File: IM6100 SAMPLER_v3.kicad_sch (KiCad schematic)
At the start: 0 parts

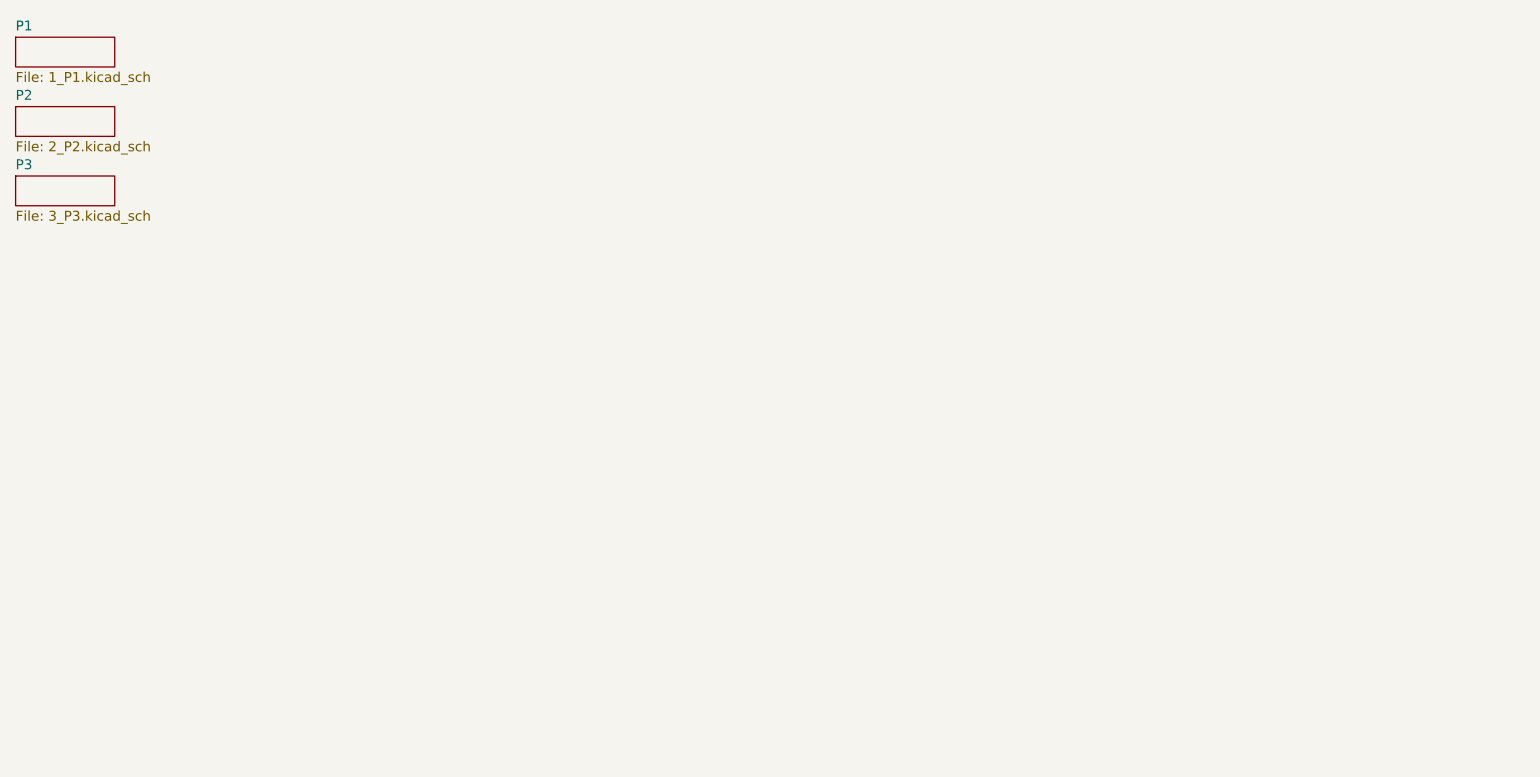
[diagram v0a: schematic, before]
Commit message: HID board finalizing
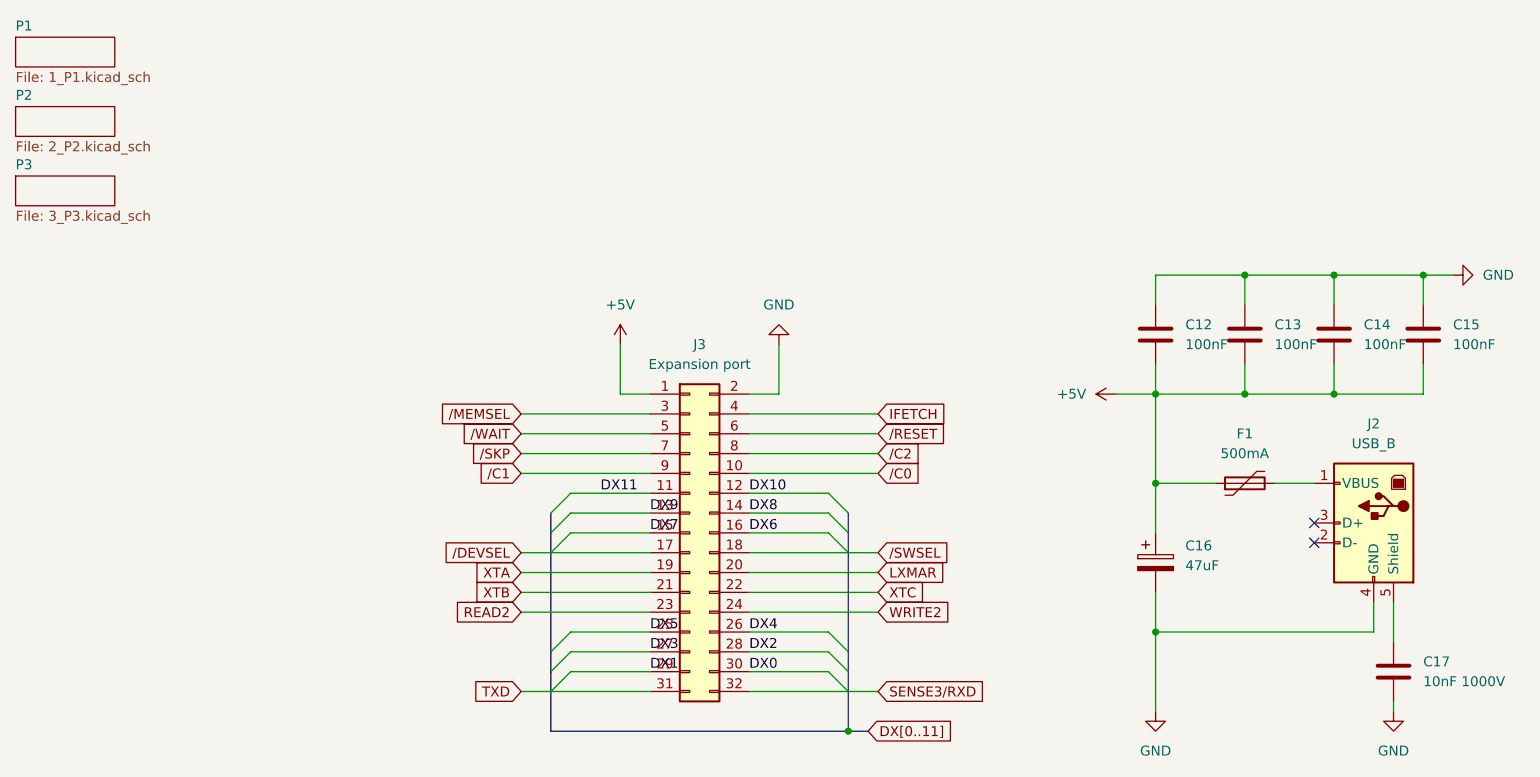
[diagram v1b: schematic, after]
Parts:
- added C12, C13, C14, C15: 100nF, Capacitor_THT:C_Disc_D5.0mm_W2.5mm_P2.50mm, symbol Device:C
- added C16: 47uF, Capacitor_THT:CP_Radial_D6.3mm_P2.50mm, symbol Device:C_Polarized
- added C17: 10nF 1000V, Capacitor_THT:C_Disc_D5.0mm_W2.5mm_P2.50mm, symbol Device:C
- added F1: 500mA, Capacitor_THT:C_Disc_D6.0mm_W2.5mm_P5.00mm, symbol Device:Polyfuse
- added J2: USB_B, Connector_USB:USB_B_Lumberg_2411_02_Horizontal, symbol Connector:USB_B
- added J3: Expansion port, Connector_PinHeader_2.54mm:PinHeader_2x16_P2.54mm_Vertical, symbol Connector_Generic:Conn_02x16_Odd_Even
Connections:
- new net: F1.2, J2.1 (VBUS)
- new net: C17.1, J2.5 (Shield)
- new net +5V: C12.2, C13.2, C14.2, C15.2, C16.1, F1.1, J3.1 (Pin_1)
- new net /C0: J3.10 (Pin_10)
- new net /C1: J3.9 (Pin_9)
- new net /C2: J3.8 (Pin_8)
- new net /DEVSEL: J3.17 (Pin_17)
- new net /MEMSEL: J3.3 (Pin_3)
- new net /SKP: J3.7 (Pin_7)
- new net /SWSEL: J3.18 (Pin_18)
- new net DX0: J3.30 (Pin_30)
- new net DX1: J3.29 (Pin_29)
- new net DX10: J3.12 (Pin_12)
- new net DX11: J3.11 (Pin_11)
- new net DX2: J3.28 (Pin_28)
- new net DX3: J3.27 (Pin_27)
- new net DX4: J3.26 (Pin_26)
- new net DX5: J3.25 (Pin_25)
- new net DX6: J3.16 (Pin_16)
- new net DX7: J3.15 (Pin_15)
- new net DX8: J3.14 (Pin_14)
- new net DX9: J3.13 (Pin_13)
- new net GND: C12.1, C13.1, C14.1, C15.1, C16.2, C17.2, J2.4 (GND), J3.2 (Pin_2)
- new net IFETCH: J3.4 (Pin_4)
- new net LXMAR: J3.20 (Pin_20)
- new net READ2: J3.23 (Pin_23)
- new net SENSE3/RXD: J3.32 (Pin_32)
- new net TXD: J3.31 (Pin_31)
- new net WRITE2: J3.24 (Pin_24)
- new net XTA: J3.19 (Pin_19)
- new net XTB: J3.21 (Pin_21)
- new net XTC: J3.22 (Pin_22)
- new net /RESET: J3.6 (Pin_6)
- new net /WAIT: J3.5 (Pin_5)
- no-connect marks 0 -> 2
